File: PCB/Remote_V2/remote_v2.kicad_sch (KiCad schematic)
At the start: 100 parts, among them J10 Yaxis J1, J11 Yaxis J2, J12 Yaxis J3, J13 Yaxis J4, J14 ICSP1, J15 ICSP2, J16 ICSP3, J18 Peri Soc 1, J19 Peri Soc 2, J2 ADS1115 A1, J20 Peri Soc 3, J21 UART Soc 1, J22 UART Soc 2, J23 UART Soc 3, J24 5V, J25 XT60-M, J26 UART RASP, J27 RASP Peripheral, J3 ADS1115 A2, J4 Xaxis J1, J7 Xaxis J2, J8 Xaxis J3, J9 Xaxis J4, Q4 BC847, Q5 BC847, Q8 BC847, Q9 BC847, SW7 SW_SPDT, SW8 SW_SPDT, U11 Ai-Thinker-Ra-02, U12 Ai-Thinker-Ra-02, U13 MPU-6050, U2 RASPBERRY_PI_4B_4GB

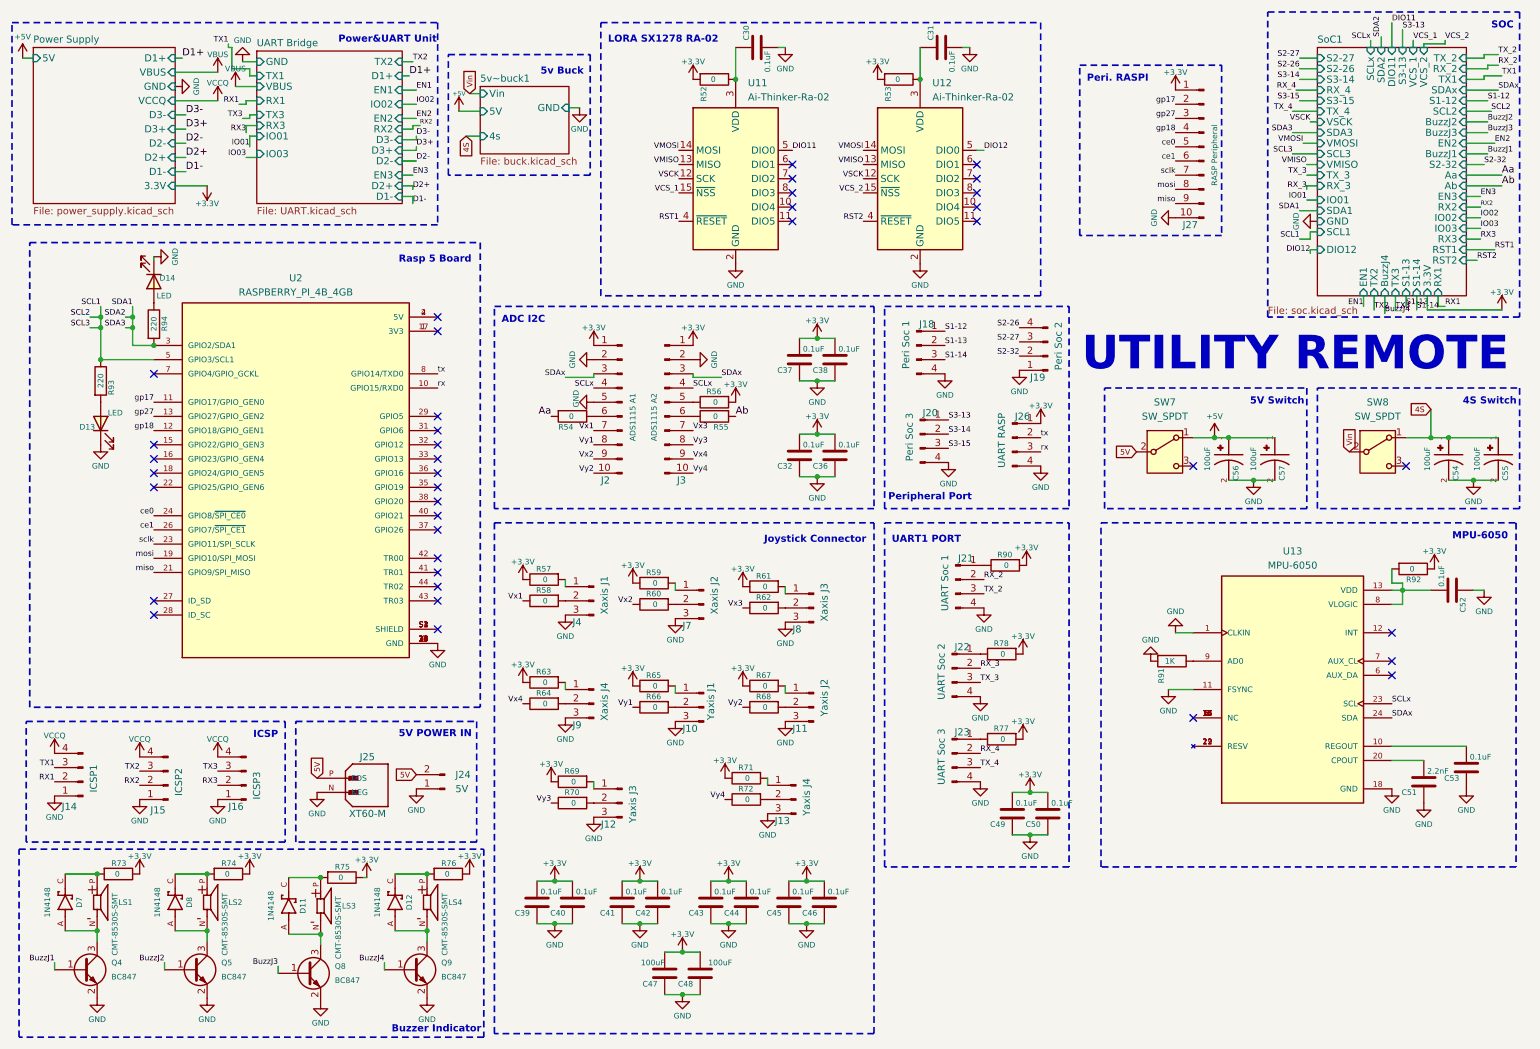
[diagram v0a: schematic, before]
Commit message: update remote_v2
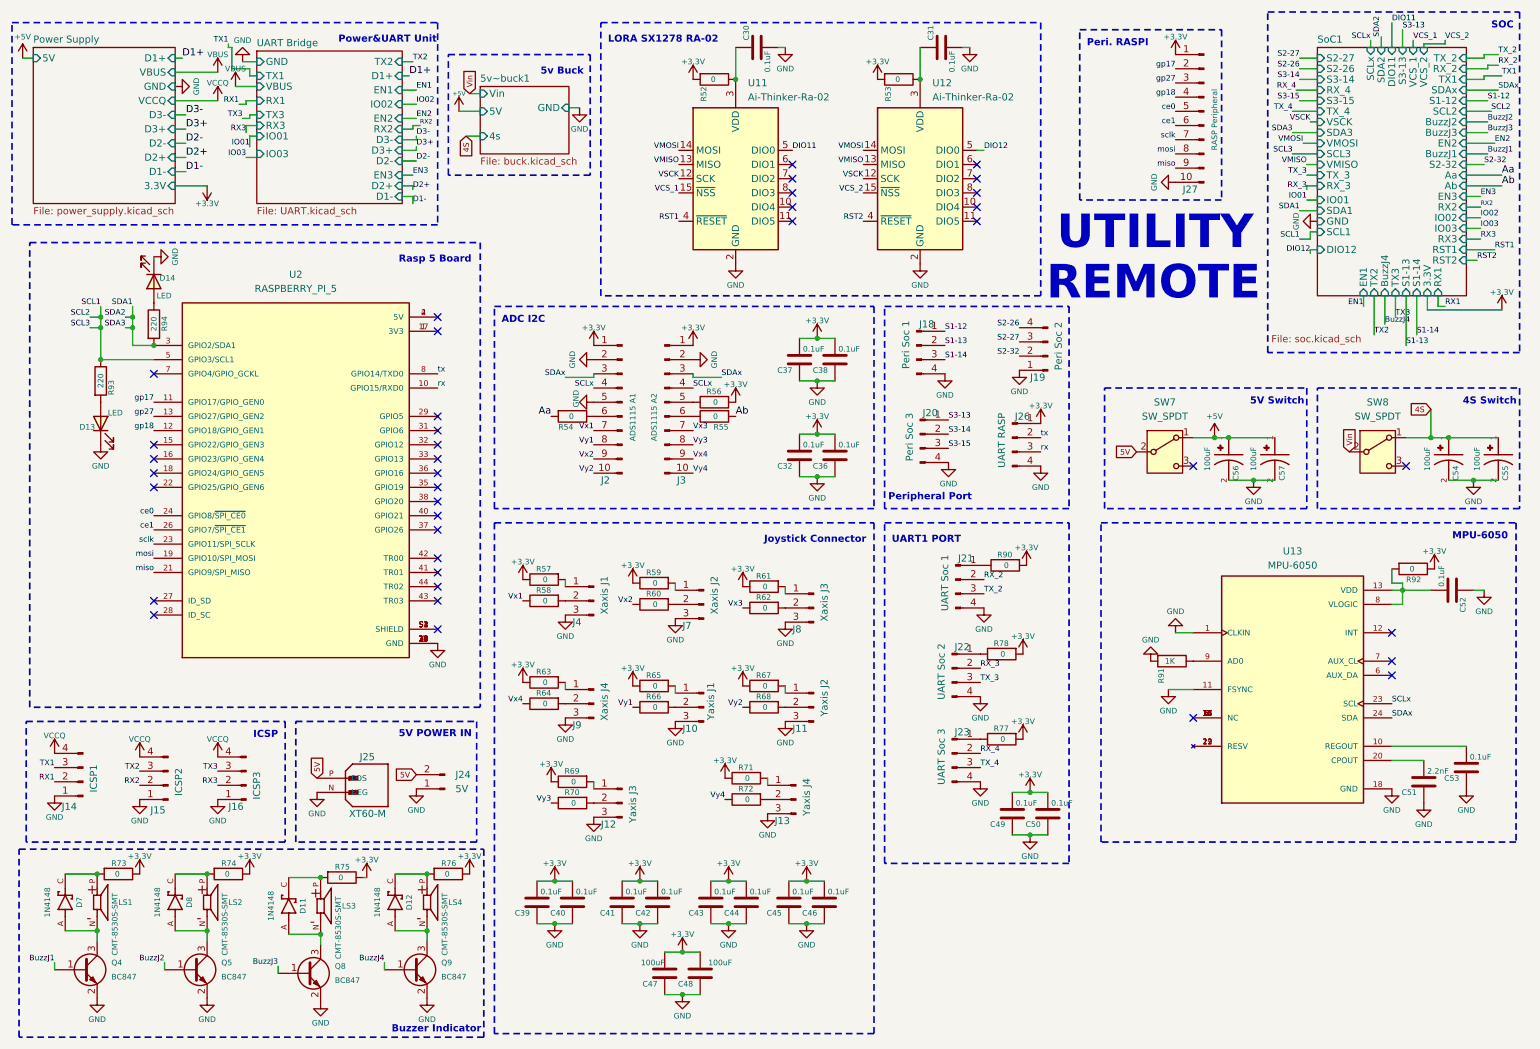
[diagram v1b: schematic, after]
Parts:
- U2: value RASPBERRY_PI_4B_4GB -> RASPBERRY_PI_5
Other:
- note added: "REMOTE"
- note added: "UTILITY"
- note removed: "UTILITY REMOTE"
- moved on the sheet: J27
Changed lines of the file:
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@@
     (stroke (width 0) (type default))
   )
-  (wire (pts (xy 257.175 63.5) (xy 257.175 66.04))
+  (wire (pts (xy 257.175 63.5) (xy 257.175 70.485))
     (stroke (width 0) (type default))
   )
@@
     (stroke (width 0) (type default))
   )
-  (wire (pts (xy 262.89 63.5) (xy 262.89 65.405))
+  (wire (pts (xy 262.89 63.5) (xy 262.89 72.39))
     (stroke (width 0) (type default))
   )
@@
     (stroke (width 0) (type default))
   )
-  (wire (pts (xy 259.08 63.5) (xy 259.08 66.675))
+  (wire (pts (xy 259.08 63.5) (xy 259.08 68.58))
     (stroke (width 0) (type default))
   )
@@
     (stroke (width 0) (type default))
   )
-  (wire (pts (xy 264.795 63.5) (xy 264.795 66.04))
+  (wire (pts (xy 264.795 63.5) (xy 264.795 70.485))
     (stroke (width 0) (type default))
   )
@@
     (stroke (width 0) (type default))
   )
-  (wire (pts (xy 260.985 63.5) (xy 260.985 66.04))
+  (wire (pts (xy 260.985 63.5) (xy 260.985 67.31))
     (stroke (width 0) (type default))
   )
@@
     (stroke (width 0) (type default))
   )
-  (rectangle (start 208.28 104.14) (end 282.575 165.735)
+  (rectangle (start 208.28 104.14) (end 282.575 161.29)
     (stroke (width 0.3) (type dash) (color 255 44 9 1))
     (fill (type none))
@@
     (fill (type none))
   )
-  (rectangle (start 169.545 104.14) (end 202.565 165.735)
+  (rectangle (start 169.545 104.14) (end 202.565 165.1)
     (stroke (width 0.3) (type dash) (color 255 44 9 1))
     (fill (type none))
@@
     (fill (type none))
   )
-  (rectangle (start 238.125 12.7) (end 283.21 67.31)
+  (rectangle (start 238.125 12.7) (end 283.21 73.66)
     (stroke (width 0.3) (type dash) (color 255 44 9 1))
     (fill (type none))
@@
     (fill (type none))
   )
-  (rectangle (start 204.47 22.225) (end 229.87 52.705)
+  (rectangle (start 204.47 15.875) (end 229.87 46.355)
     (stroke (width 0.3) (type dash) (color 255 44 9 1))
     (fill (type none))
@@
     (fill (type none))
   )
-  (text "UTILITY REMOTE\n" (at 281.305 77.47 0)
+  (text "UTILITY\n\n" (at 235.585 65.405 0)
     (effects (font (size 6 6) (thickness 1.6) bold (color 253 61 255 1)) (justify right bottom))
   )
@@
     (effects (font (size 1.27 1.27) bold (color 0 28 255 1)) (justify left bottom))
   )
-  (text "Peri. RASPI\n" (at 205.74 25.4 0)
+  (text "Peri. RASPI\n" (at 205.74 19.05 0)
     (effects (font (size 1.27 1.27) bold (color 0 28 255 1)) (justify left bottom))
   )
@@
     (effects (font (size 1.27 1.27) bold (color 0 28 255 1)) (justify left bottom))
   )
+  (text "\nREMOTE\n" (at 236.855 64.77 0)
+    (effects (font (size 6 6) (thickness 1.6) bold (color 253 61 255 1)) (justify right bottom))
+  )
   (text "ICSP\n" (at 56.515 142.875 0)
     (effects (font (size 1.27 1.27) bold (color 0 28 255 1)) (justify left bottom))
@@
     (effects (font (size 1.27 1.27)) (justify left bottom))
   )
-  (label "ce0" (at 221.615 36.83 180) (fields_autoplaced)
+  (label "ce0" (at 221.615 30.48 180) (fields_autoplaced)
     (effects (font (size 1 1)) (justify right bottom))
   )
@@
     (effects (font (size 1 1)) (justify right bottom))
   )
-  (label "ce1" (at 221.615 39.37 180) (fields_autoplaced)
+  (label "ce1" (at 221.615 33.02 180) (fields_autoplaced)
     (effects (font (size 1 1)) (justify right bottom))
   )
@@
     (effects (font (size 1 1)) (justify right bottom))
   )
-  (label "BuzzJ4" (at 259.08 66.675 0) (fields_autoplaced)
+  (label "BuzzJ4" (at 259.08 68.58 0) (fields_autoplaced)
     (effects (font (size 1 1)) (justify left bottom))
   )
@@
     (effects (font (size 1 1)) (justify left bottom))
   )
-  (label "sclk" (at 221.615 41.91 180) (fields_autoplaced)
+  (label "sclk" (at 221.615 35.56 180) (fields_autoplaced)
     (effects (font (size 1 1)) (justify right bottom))
   )
@@
     (effects (font (size 1 1)) (justify right bottom))
   )
-  (label "S1-14" (at 264.795 66.04 0) (fields_autoplaced)
+  (label "S1-14" (at 264.795 70.485 0) (fields_autoplaced)
     (effects (font (size 1 1)) (justify left bottom))
   )
@@
     (effects (font (size 1 1)) (justify left bottom))
   )
-  (label "miso" (at 221.615 46.99 180) (fields_autoplaced)
+  (label "miso" (at 221.615 40.64 180) (fields_autoplaced)
     (effects (font (size 1 1)) (justify right bottom))
   )
@@
     (effects (font (size 1 1)) (justify right bottom))
   )
-  (label "S1-13" (at 262.89 65.405 0) (fields_autoplaced)
+  (label "S1-13" (at 262.89 72.39 0) (fields_autoplaced)
     (effects (font (size 1 1)) (justify left bottom))
   )
@@
     (effects (font (size 1 1)) (justify left bottom))
   )
-  (label "TX2" (at 257.175 66.04 0) (fields_autoplaced)
+  (label "TX2" (at 257.175 70.485 0) (fields_autoplaced)
     (effects (font (size 1 1)) (justify left bottom))
   )
@@
     (effects (font (size 1 1)) (justify right bottom))
   )
-  (label "gp17" (at 221.615 29.21 180) (fields_autoplaced)
+  (label "gp17" (at 221.615 22.86 180) (fields_autoplaced)
     (effects (font (size 1 1)) (justify right bottom))
   )
@@
     (effects (font (size 1.27 1.27)) (justify left bottom))
   )
-  (label "TX3" (at 260.985 66.04 0) (fields_autoplaced)
+  (label "TX3" (at 260.985 67.31 0) (fields_autoplaced)
     (effects (font (size 1 1)) (justify left bottom))
   )
@@
     (effects (font (size 1.27 1.27)) (justify left bottom))
   )
-  (label "gp18" (at 221.615 34.29 180) (fields_autoplaced)
+  (label "gp18" (at 221.615 27.94 180) (fields_autoplaced)
     (effects (font (size 1 1)) (justify right bottom))
   )
@@
     (effects (font (size 1 1)) (justify right bottom))
   )
-  (label "gp27" (at 221.615 31.75 180) (fields_autoplaced)
+  (label "gp27" (at 221.615 25.4 180) (fields_autoplaced)
     (effects (font (size 1 1)) (justify right bottom))
   )
@@
     (effects (font (size 1 1)) (justify right bottom))
   )
-  (label "mosi" (at 221.615 44.45 180) (fields_autoplaced)
+  (label "mosi" (at 221.615 38.1 180) (fields_autoplaced)
     (effects (font (size 1 1)) (justify right bottom))
   )
@@
     )
   )
-  (symbol (lib_id "power:GND") (at 221.615 49.53 270) (unit 1)
+  (symbol (lib_id "power:GND") (at 221.615 43.18 270) (unit 1)
     (in_bom yes) (on_board yes) (dnp no)
-    (property "Reference" "#PWR0207" (at 215.265 49.53 0)
+    (property "Reference" "#PWR0207" (at 215.265 43.18 0)
       (effects (font (size 1.27 1.27)) hide)
     )
-    (property "Value" "GND" (at 217.805 49.53 0)
+    (property "Value" "GND" (at 217.805 43.18 0)
       (effects (font (size 1 1)))
     )
-    (property "Footprint" "" (at 221.615 49.53 0)
+    (property "Footprint" "" (at 221.615 43.18 0)
       (effects (font (size 1.27 1.27)) hide)
     )
-    (property "Datasheet" "" (at 221.615 49.53 0)
+    (property "Datasheet" "" (at 221.615 43.18 0)
       (effects (font (size 1.27 1.27)) hide)
     )
@@
     )
   )
-  (symbol (lib_id "Connector:Conn_01x10_Pin") (at 226.695 36.83 0) (mirror y) (unit 1)
+  (symbol (lib_id "Connector:Conn_01x10_Pin") (at 226.695 30.48 0) (mirror y) (unit 1)
     (in_bom yes) (on_board yes) (dnp no)
-    (property "Reference" "J27" (at 222.885 50.8 0)
+    (property "Reference" "J27" (at 222.885 44.45 0)
       (effects (font (size 1.27 1.27)) (justify right))
     )
-    (property "Value" "RASP Peripheral" (at 228.6 43.815 90)
+    (property "Value" "RASP Peripheral" (at 228.6 37.465 90)
       (effects (font (size 1 1)) (justify left))
     )
-    (property "Footprint" "Connector_PinHeader_2.54mm:PinHeader_1x10_P2.54mm_Vertical" (at 226.695 36.83 0)
+    (property "Footprint" "Connector_PinHeader_2.54mm:PinHeader_1x10_P2.54mm_Vertical" (at 226.695 30.48 0)
       (effects (font (size 1.27 1.27)) hide)
     )
-    (property "Datasheet" "~" (at 226.695 36.83 0)
+    (property "Datasheet" "~" (at 226.695 30.48 0)
       (effects (font (size 1.27 1.27)) hide)
     )
@@
   (symbol (lib_id "RASPBERRY_PI_4B:RASPBERRY_PI_4B_4GB") (at 64.135 97.79 0) (unit 1)
     (in_bom yes) (on_board yes) (dnp no) (fields_autoplaced)
-    (property "Reference" "U2" (at 64.135 60.325 0)
+    (property "Reference" "U2" (at 64.135 59.69 0)
       (effects (font (size 1.27 1.27)))
     )
-    (property "Value" "RASPBERRY_PI_4B_4GB" (at 64.135 62.865 0)
+    (property "Value" "RASPBERRY_PI_5" (at 64.135 62.23 0)
       (effects (font (size 1.27 1.27)))
     )
@@
     )
   )
-  (symbol (lib_id "power:+3.3V") (at 221.615 26.67 0) (mirror y) (unit 1)
+  (symbol (lib_id "power:+3.3V") (at 221.615 20.32 0) (mirror y) (unit 1)
     (in_bom yes) (on_board yes) (dnp no)
-    (property "Reference" "#PWR0206" (at 221.615 30.48 0)
+    (property "Reference" "#PWR0206" (at 221.615 24.13 0)
       (effects (font (size 1.27 1.27)) hide)
     )
-    (property "Value" "+3.3V" (at 221.615 23.495 0)
+    (property "Value" "+3.3V" (at 221.615 17.145 0)
       (effects (font (size 1 1)))
     )
-    (property "Footprint" "" (at 221.615 26.67 0)
+    (property "Footprint" "" (at 221.615 20.32 0)
       (effects (font (size 1.27 1.27)) hide)
     )
-    (property "Datasheet" "" (at 221.615 26.67 0)
+    (property "Datasheet" "" (at 221.615 20.32 0)
       (effects (font (size 1.27 1.27)) hide)
     )
@@
       (effects (font (size 1.27 1.27)) (justify left bottom))
     )
-    (property "Sheetfile" "soc.kicad_sch" (at 238.125 65.405 0)
+    (property "Sheetfile" "soc.kicad_sch" (at 238.76 70.485 0)
       (effects (font (size 1.27 1.27)) (justify left top))
     )
